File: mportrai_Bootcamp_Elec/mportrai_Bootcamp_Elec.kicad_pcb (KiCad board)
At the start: 2 copper layers, 22.8 x 33.1 mm, 17 parts, among them J3 FTDI, SW1 SW_Push, U1 ATmega328P-A, Y1 16MHz

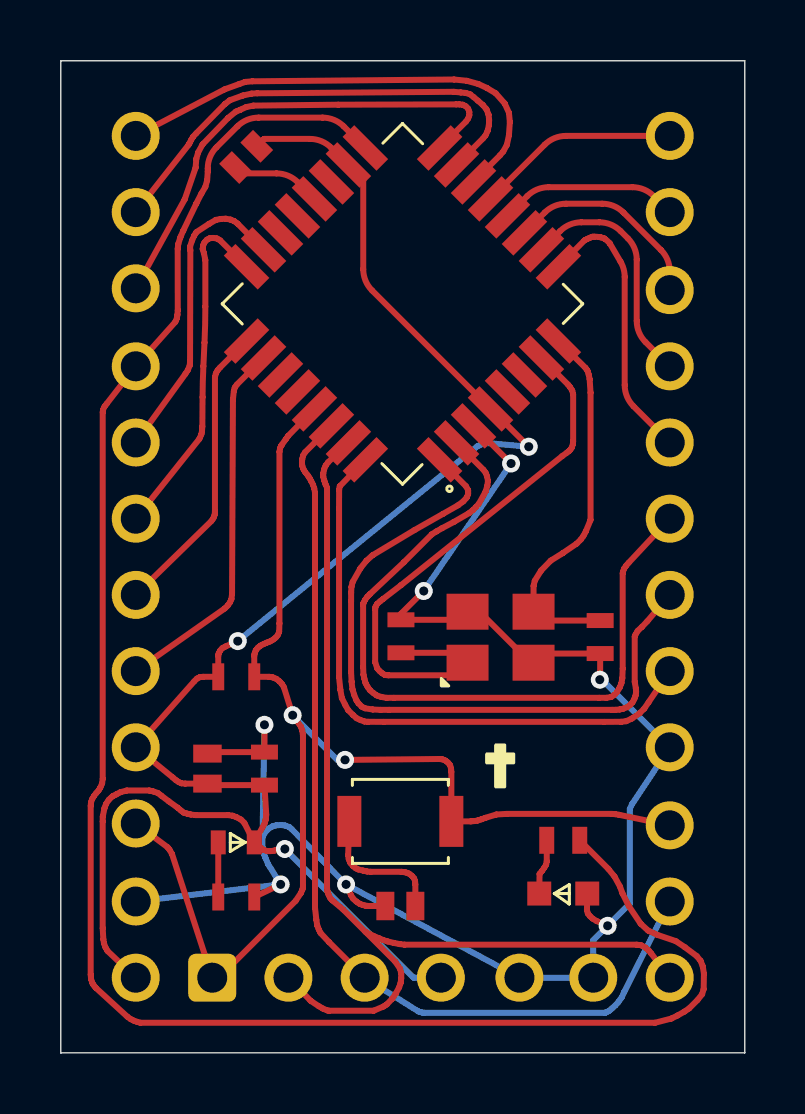
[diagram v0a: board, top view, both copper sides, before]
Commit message: modif sch-pcb, modif librairie * to mportrai_*, pinout
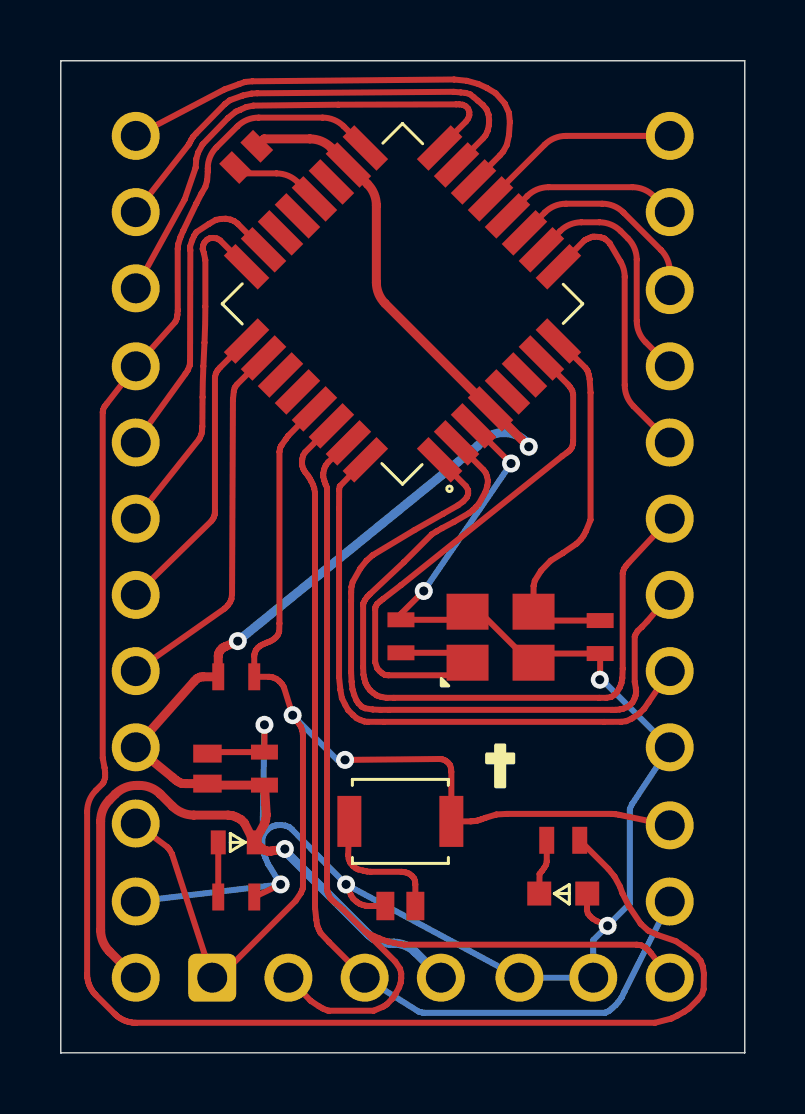
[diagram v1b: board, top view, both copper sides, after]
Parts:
- C1, C2: footprint my_footprints:CL10C120JB8NNNC -> mportrai_footprints:CL10C120JB8NNNC
- C3, C4, C7: footprint my_footprints:CC0603KRX7R9BB104 -> mportrai_footprints:CC0603KRX7R9BB104
- C6: footprint my_footprints:CL10A105KB8NNNC -> mportrai_footprints:CL10A105KB8NNNC
- D1: footprint my_footprints:TZ-P2-0603YGTCS1-0.6T -> mportrai_footprints:TZ-P2-0603YGTCS1-0.6T
- D2: footprint my_footprints:XL-1608SURC-06 -> mportrai_footprints:XL-1608SURC-06
- J1, J2: footprint my_footprints:Connecteur_1 -> mportrai_footprints:Connecteur_1
- J3: footprint my_footprints:Connecteur_2 -> mportrai_footprints:Connecteur_2
- R1: footprint my_footprints:0603WAF3300T5E -> mportrai_footprints:0603WAF3300T5E
- R2, R3: footprint my_footprints:RC0603FR-0710KL -> mportrai_footprints:RC0603FR-0710KL
- SW1: footprint my_footprints:B3U-1000P -> mportrai_footprints:B3U-1000P
- U1: footprint my_footprints:ATMEGA328P-AU -> mportrai_footprints:ATMEGA328P-AU
- Y1: footprint my_footprints:X322516MLB4SI -> mportrai_footprints:X322516MLB4SI
